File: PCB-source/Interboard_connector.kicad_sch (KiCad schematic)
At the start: 1 part, among them J1 86093488324755V1LF

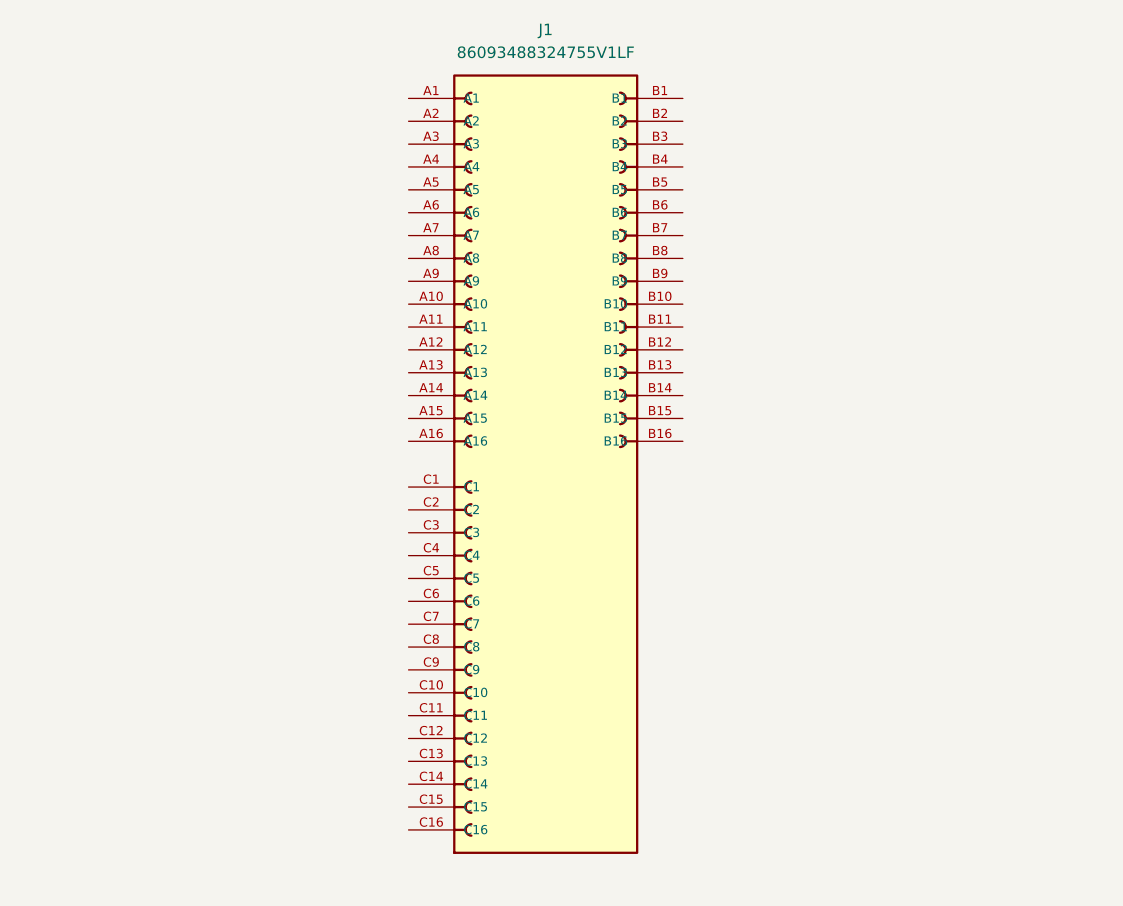
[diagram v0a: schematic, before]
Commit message: in progress
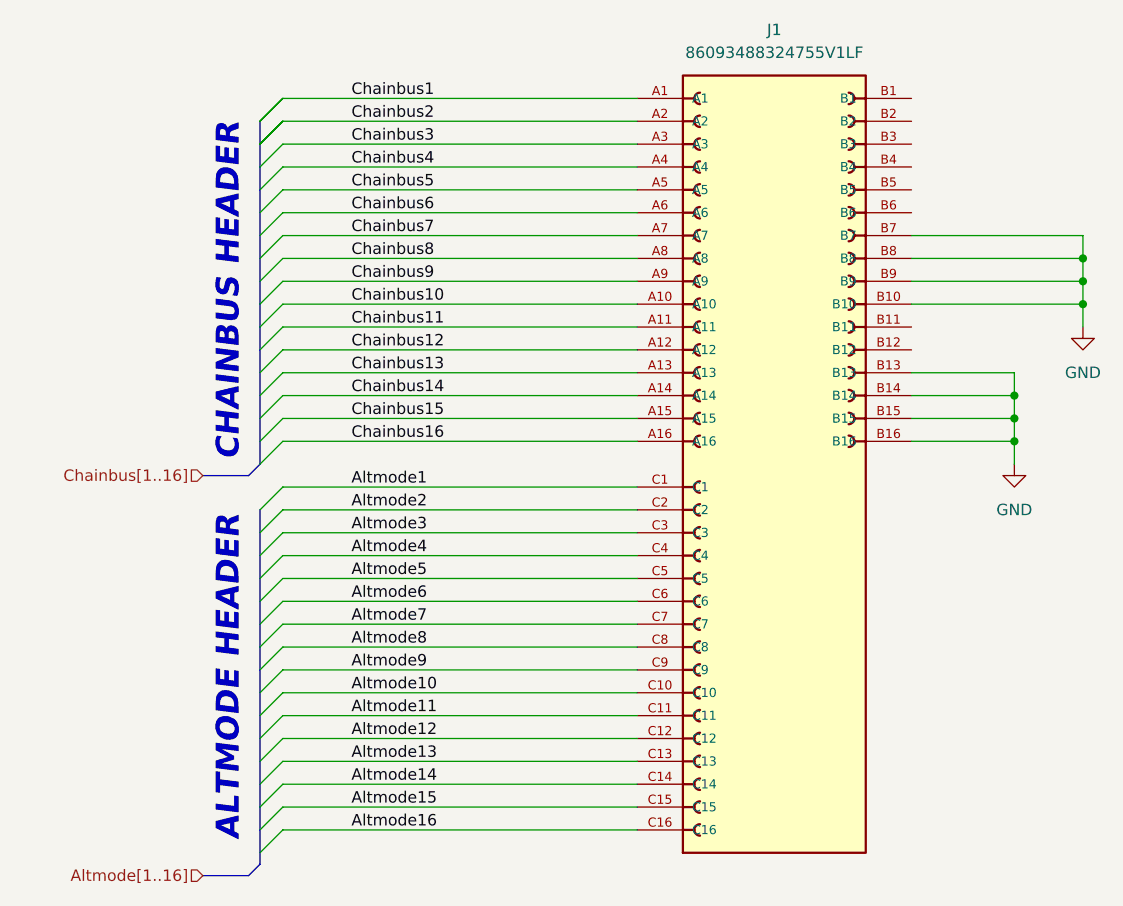
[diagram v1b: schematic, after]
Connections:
- net Chainbus1: now reaches J1.A1
- net Chainbus10: now reaches J1.A10
- net Chainbus11: now reaches J1.A11
- net Chainbus12: now reaches J1.A12
- net Chainbus13: now reaches J1.A13
- net Chainbus14: now reaches J1.A14
- net Chainbus15: now reaches J1.A15
- net Chainbus16: now reaches J1.A16
- net Chainbus2: now reaches J1.A2
- net Chainbus3: now reaches J1.A3
- net Chainbus4: now reaches J1.A4
- net Chainbus5: now reaches J1.A5
- net Chainbus6: now reaches J1.A6
- net Chainbus7: now reaches J1.A7
- net Chainbus8: now reaches J1.A8
- net Chainbus9: now reaches J1.A9
- net GND: now reaches J1.B10
- net GND: now also J1.B13, J1.B14, J1.B15, J1.B16, J1.B7, J1.B8, J1.B9
- net Altmode1: now reaches J1.C1
- net Altmode10: now reaches J1.C10
- net Altmode11: now reaches J1.C11
- net Altmode12: now reaches J1.C12
- net Altmode13: now reaches J1.C13
- net Altmode14: now reaches J1.C14
- net Altmode15: now reaches J1.C15
- net Altmode16: now reaches J1.C16
- net Altmode2: now reaches J1.C2
- net Altmode3: now reaches J1.C3
- net Altmode4: now reaches J1.C4
- net Altmode5: now reaches J1.C5
- net Altmode6: now reaches J1.C6
- net Altmode7: now reaches J1.C7
- net Altmode8: now reaches J1.C8
- net Altmode9: now reaches J1.C9
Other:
- note added: "ALTMODE HEADER"
- note added: "CHAINBUS HEADER"
- moved on the sheet: J1
